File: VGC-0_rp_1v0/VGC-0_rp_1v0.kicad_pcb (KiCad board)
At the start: 4 copper layers, 51 x 82 mm, 99 parts, among them J2 THT pins for BATTERY, J3 SMD pads for 3.3V, J4 SM03B-SRSS-TB, SW1 SW_Push, SW2 SW_Push, SW3 SW_Push, SW4 SW_Push, U1 RP2350_60QFN, U2 RT6154A, U3 W25Q128JVS, U4 ESP8684-MINI-1, U5 APS1604M-3SQR-ZR, U7 BQ24073RGTR, Y1 ABM8-272-T3

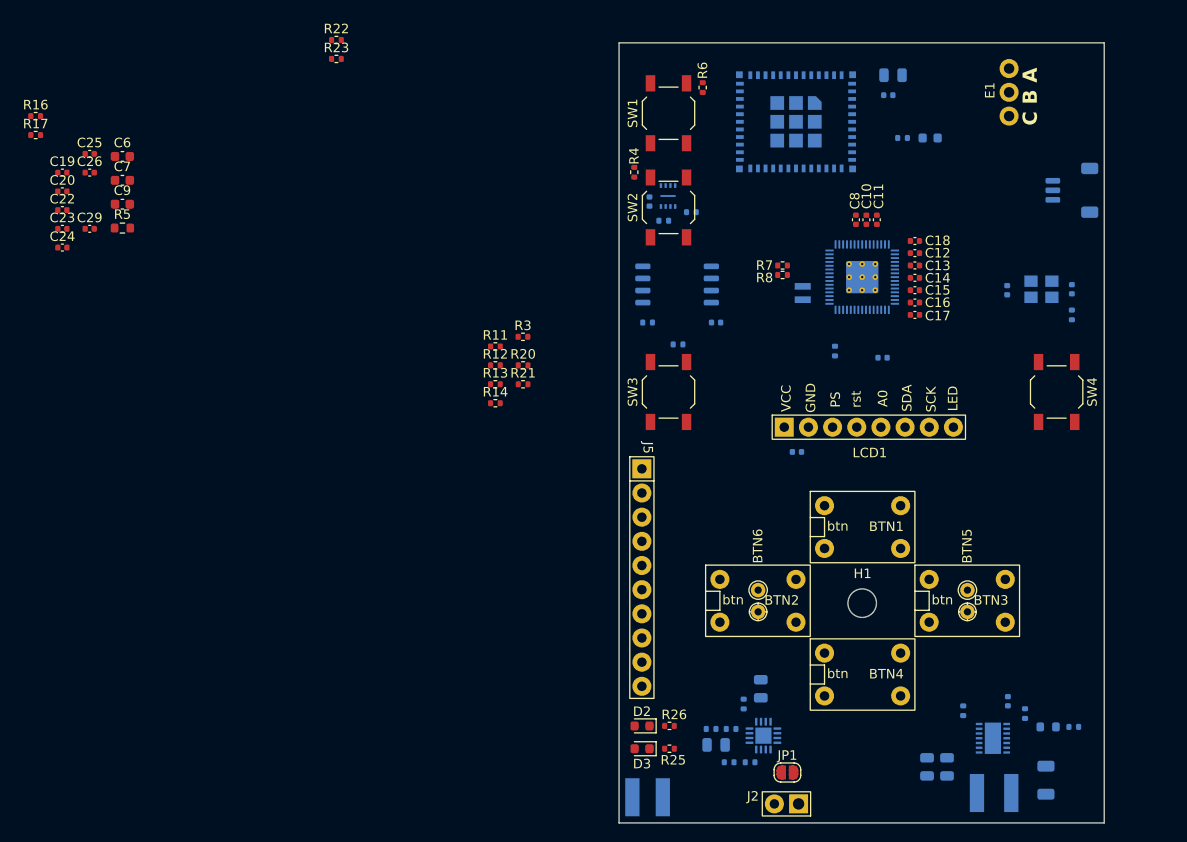
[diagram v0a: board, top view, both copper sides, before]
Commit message: update rev.2.2
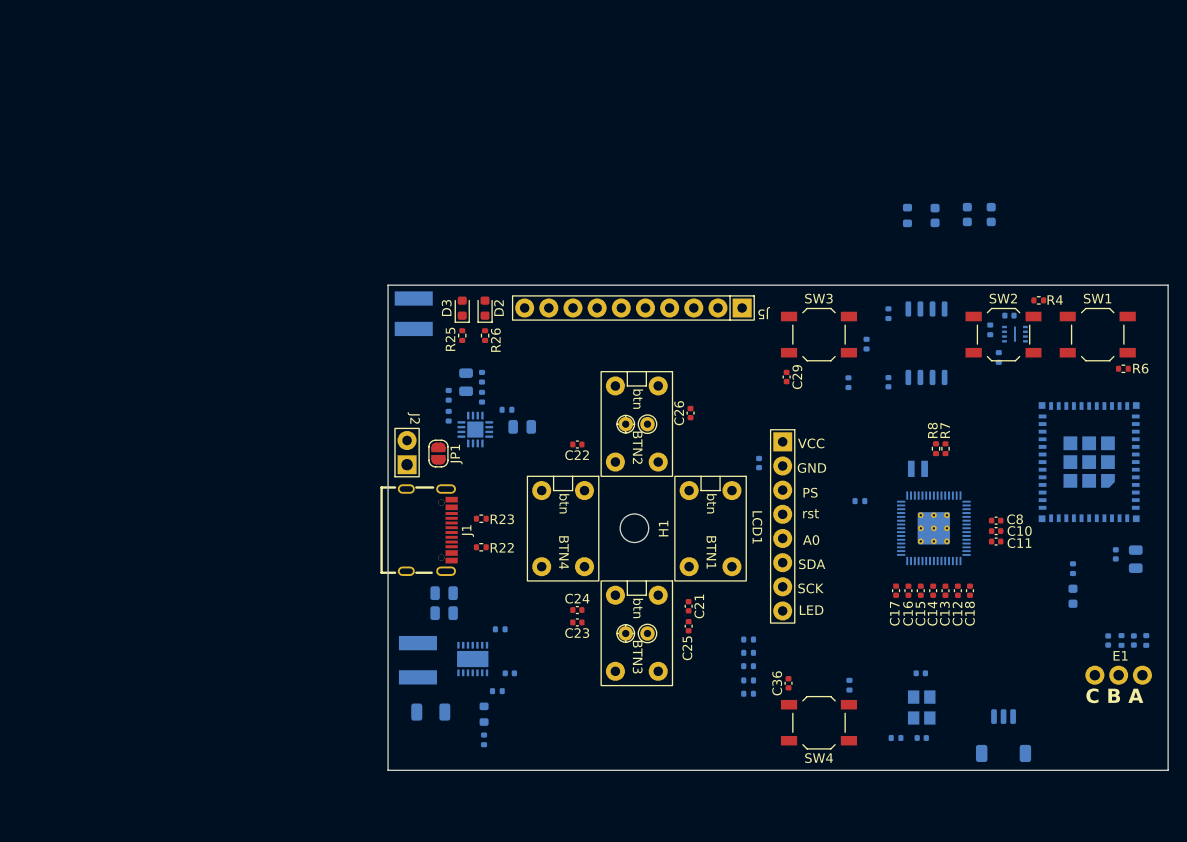
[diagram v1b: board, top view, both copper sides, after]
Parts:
- added C36: 2.2u, Capacitor_SMD:C_0402_1005Metric, F.Cu at (161.2, 118.4)
- added J1: USB-TYPE-C-017, our-parts:USB-TYPE-C-SMD_C9900008089, F.Cu at (123.4, 102.3)
- BTN5, BTN6, C19, C20, C6, C7, C9, R11, R12, R13, R14, R16, R17, R20, R21, R3, R5: moved to B.Cu
- C21: moved to F.Cu
- moved R16 129.1 mm to (198.8, 113.9), turned to -90 degrees
- moved R17 125.9 mm to (196.2, 113.9), turned to -90 degrees
- moved C19 122.9 mm to (197.5, 113.9), turned to 90 degrees
- moved C20 119.6 mm to (194.8, 113.9), turned to 90 degrees
- moved C6 91.5 mm to (182.5, 69.1), turned to 90 degrees
- moved C7 88.9 mm to (180.0, 69.1), turned to 90 degrees
- moved C9 85.4 mm to (176.6, 69.2), turned to 90 degrees
- moved R5 82.5 mm to (173.7, 69.2), turned to 90 degrees
- moved C25 80.2 mm to (150.7, 112.4), turned to 90 degrees
- moved C29 74.9 mm to (161.0, 86.2), turned to -90 degrees
- moved C23 68.1 mm to (139.0, 112.0), turned to 180 degrees
- moved C26 68.0 mm to (150.9, 90.0), turned to 90 degrees
- moved C24 66.2 mm to (139.0, 110.7)
- moved C32 65.1 mm to (123.6, 121.4), turned to 180 degrees
- moved E1 62.3 mm to (195.9, 117.6), turned to 0 degrees
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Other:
- board size 51 x 82 mm -> 82 x 51 mm
